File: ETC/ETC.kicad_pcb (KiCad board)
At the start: 2 copper layers, 96.5 x 100.5 mm, 36 parts, among them P1 DTM1312PC12PDR008, U1 NUCLEO-F446RE, U2 MCP6004, U3 LM7805_TO220, U4 LM7809_TO220, U5 ISO1050DUB, U6 ISO1050DUB, U7 SN74AHC14N

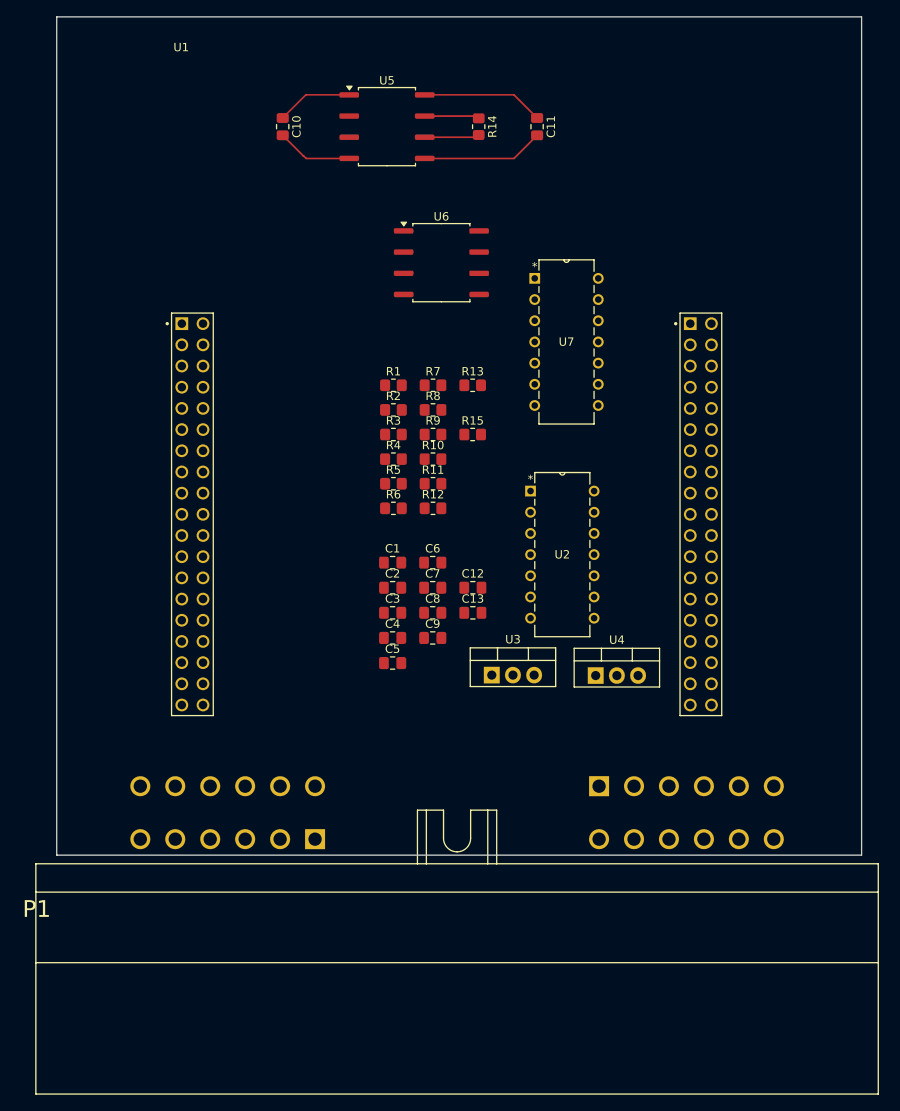
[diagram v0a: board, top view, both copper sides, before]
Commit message: did the pcb design
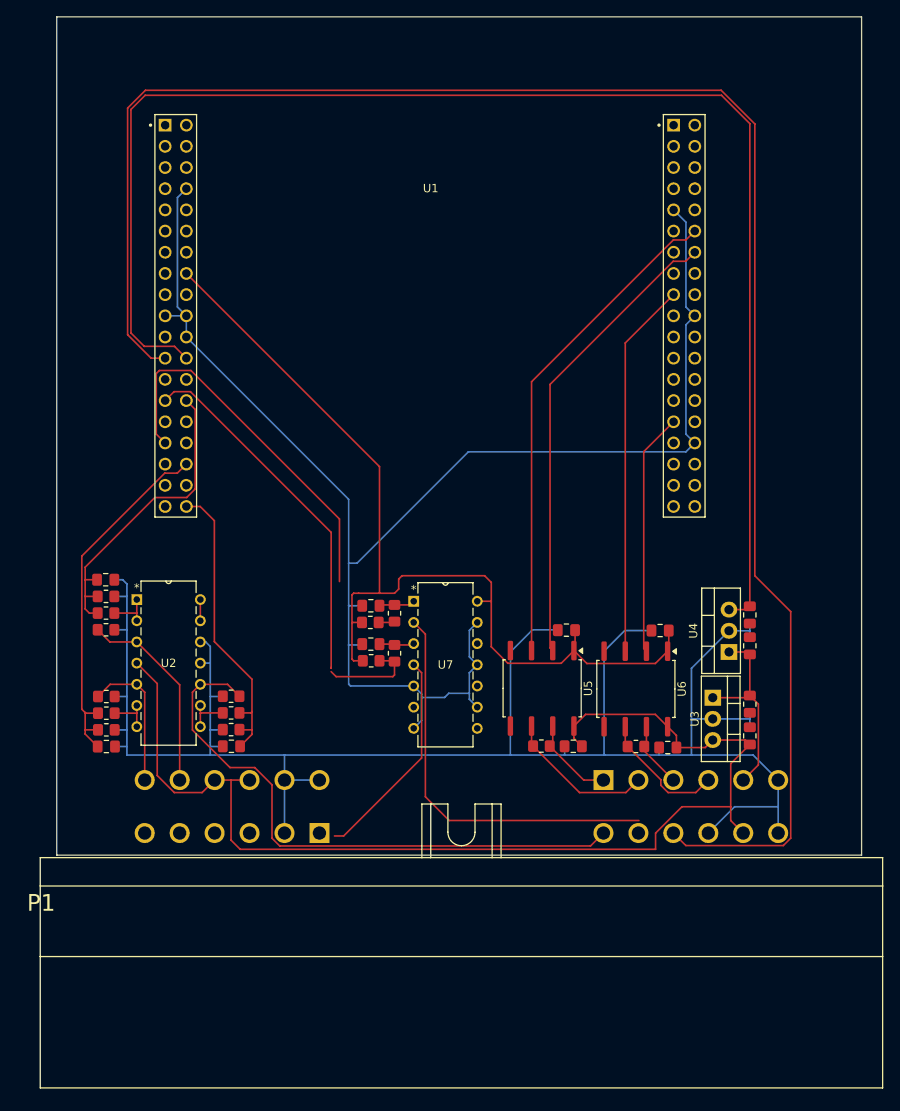
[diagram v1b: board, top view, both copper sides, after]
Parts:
- moved R14 74.6 mm to (209.1, 148.9), turned to 180 degrees
- moved C11 74.4 mm to (212.9, 148.9), turned to 180 degrees
- moved U5 69.9 mm to (209.2, 142.0), turned to -90 degrees
- moved C10 69.3 mm to (212.1, 135.0), turned to 180 degrees
- moved U6 56.2 mm to (220.4, 142.1), turned to -90 degrees
- moved U2 49.0 mm to (168.2, 146.6)
- moved C2 46.4 mm to (234.1, 147.7), turned to 90 degrees
- moved C1 46.1 mm to (234.1, 143.9), turned to -90 degrees
- moved C6 44.9 mm to (156.9, 149.0)
- moved R4 44.7 mm to (156.9, 143.0)
- moved R7 44.5 mm to (171.9, 142.9), turned to 180 degrees
- moved R5 44.1 mm to (156.9, 145.0), turned to 180 degrees
- moved R1 44.0 mm to (156.9, 133.0), turned to 180 degrees
- moved R8 43.7 mm to (171.9, 144.9)
- moved R6 43.5 mm to (156.9, 147.0)
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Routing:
- net GND: track 23.7 -> 411.9 mm
- net /RTDS: track 0.00 -> 213.1 mm
- net +9V: track 0.00 -> 171.5 mm
- net +5V: track 14.6 -> 137.6 mm
- net +3V3: track 9.12 -> 115.2 mm
- net /Cockpit_Signal: track 0.00 -> 94.0 mm
- net /BSE_RAW: track 0.00 -> 70.6 mm
- net /Reverse_Signal: track 0.00 -> 69.6 mm
- net /Motor_CAN_TD: track 0.00 -> 59.3 mm
- net /Motor_CAN_RD: track 0.00 -> 56.0 mm
- net /CAN_TD: track 0.00 -> 45.2 mm
- net /HE2: track 0.00 -> 43.8 mm
- net /HE1: track 0.00 -> 37.8 mm
- net /BSE: track 0.00 -> 36.6 mm
- net /CAN_RD: track 0.00 -> 29.1 mm
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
